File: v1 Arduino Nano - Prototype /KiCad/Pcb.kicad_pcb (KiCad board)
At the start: 2 copper layers, 4 parts

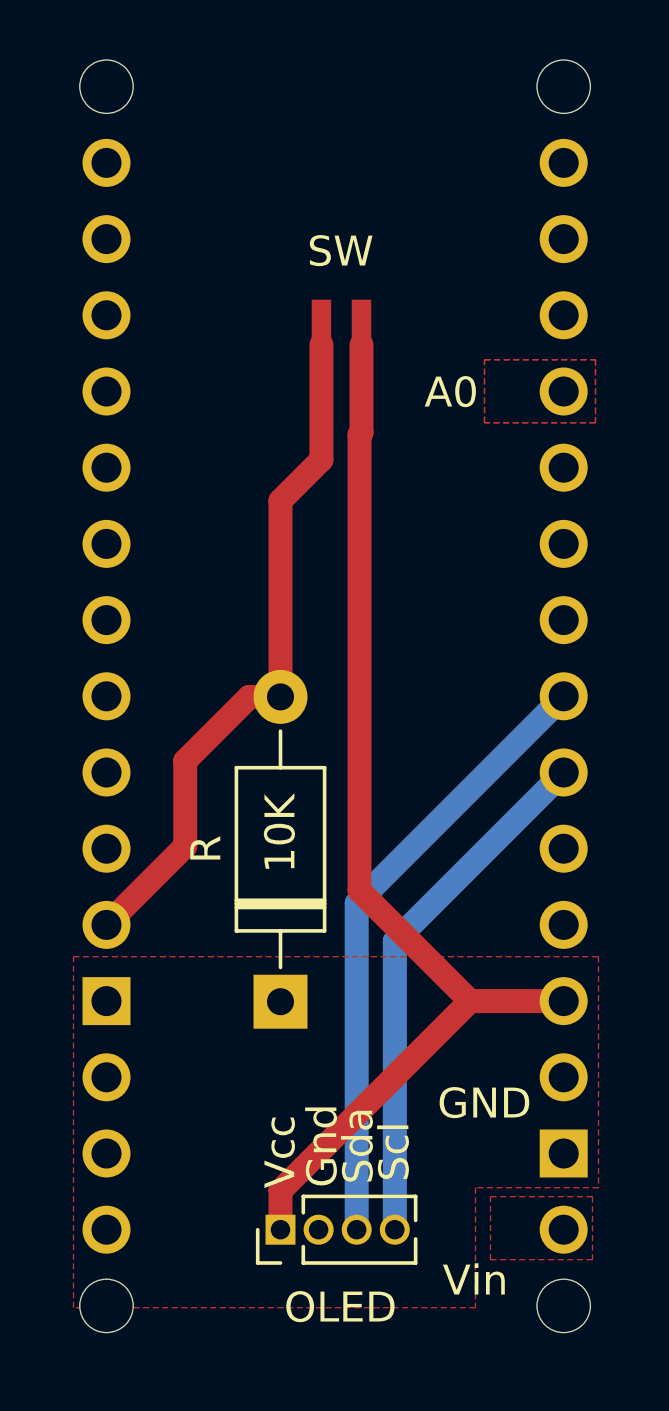
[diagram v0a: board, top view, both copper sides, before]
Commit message: update
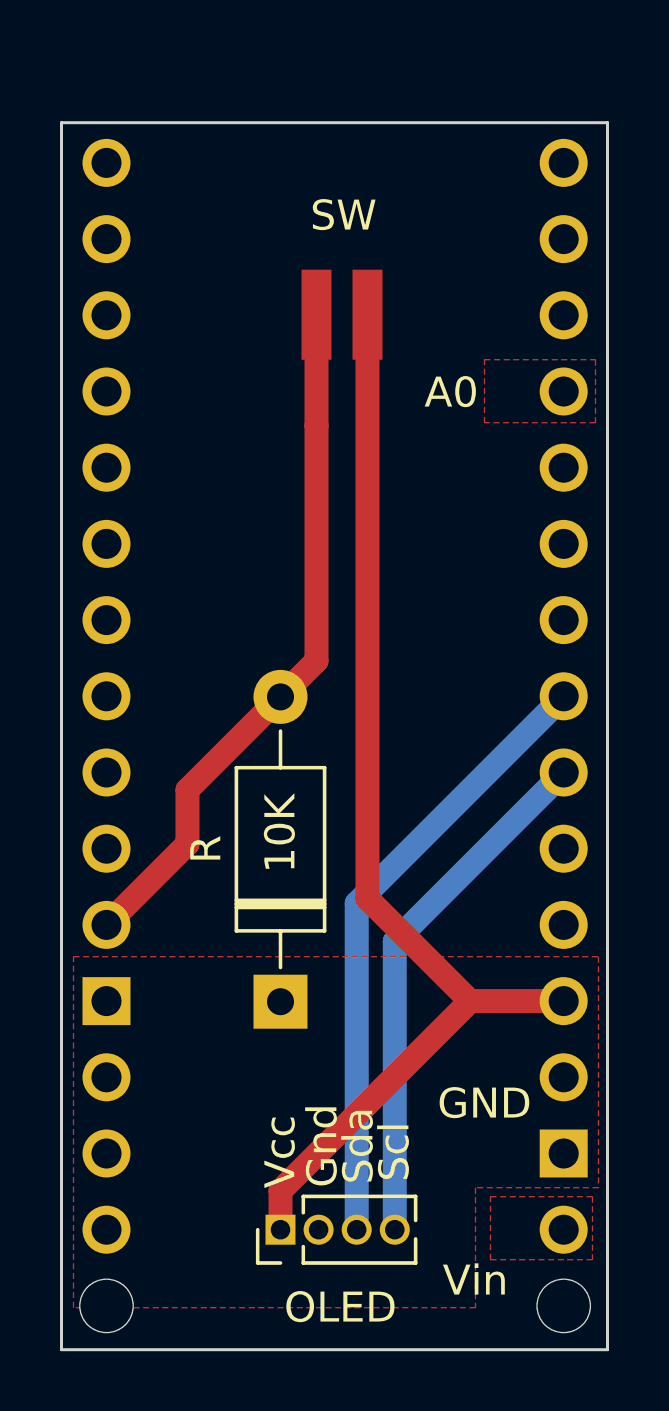
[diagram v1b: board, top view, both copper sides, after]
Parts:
- moved SW 4.00 mm to (180.7, 64.2), turned to -90 degrees
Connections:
- SW pad 1: Net-(A1-Pad5) -> /ARD5V
- SW pad 2: /ARD5V -> Net-(A1-Pad5)
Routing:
- net /ARD5V: track 36.8 -> 37.7 mm
- removed copper zone on F.Cu, net (none)
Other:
- board outline added: 18.2 x 40.9 mm
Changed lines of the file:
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@@
   )
   (module "Connector_PinHeader_1.27mm:PinHeader_1x02_P1.27mm_Vertical_SMD_Pin1Right" (layer "F.Cu")
-    (at 180.6 68.2 90)
+    (at 180.7 64.2 -90)
     (descr "surface-mounted straight pin header, 1x02, 1.27mm pitch, single row, style 2 (pin 1 right)")
     (tags "Surface mounted pin header SMD 1x02 1.27mm single row style2 pin1 right")
@@
     (property "Sheet name" "")
     (attr smd)
-    (fp_text reference "SW" (at 4.6 0) (layer "F.SilkS")
+    (fp_text reference "SW" (at -1.8 0) (layer "F.SilkS")
       (effects (font (size 1 1) (thickness 0.15)))
     )
@@
     (fp_line (start -3.5 1.8) (end 3.5 1.8) (layer "F.CrtYd") (width 0.05))
     (fp_line (start 3.5 1.8) (end 3.5 -1.8) (layer "F.CrtYd") (width 0.05))
+    (fp_line (start 3.5 -1.8) (end -3.5 -1.8) (layer "F.CrtYd") (width 0.05))
     (fp_line (start -3.5 -1.8) (end -3.5 1.8) (layer "F.CrtYd") (width 0.05))
-    (fp_line (start 3.5 -1.8) (end -3.5 -1.8) (layer "F.CrtYd") (width 0.05))
+    (fp_line (start 1.05 -0.835) (end 2.5 -0.835) (layer "F.Fab") (width 0.1))
+    (fp_line (start 2.5 -0.435) (end 1.05 -0.435) (layer "F.Fab") (width 0.1))
     (fp_line (start 2.5 -0.835) (end 2.5 -0.435) (layer "F.Fab") (width 0.1))
-    (fp_line (start 2.5 -0.435) (end 1.05 -0.435) (layer "F.Fab") (width 0.1))
-    (fp_line (start 1.05 -0.835) (end 2.5 -0.835) (layer "F.Fab") (width 0.1))
-    (pad "1" connect rect (at 1.5 -0.635 90) (size 3 0.65) (layers "F.Cu" "F.Mask")
-      (net 6 "Net-(A1-Pad5)") (pinfunction "1"))
-    (pad "2" connect rect (at 1.5 0.7 90) (size 3 0.65) (layers "F.Cu" "F.Mask")
-      (net 3 "/ARD5V") (pinfunction "2"))
+    (pad "1" connect rect (at 1.5 -0.8 270) (size 3 1) (layers "F.Cu" "F.Mask")
+      (net 3 "/ARD5V") (pinfunction "1"))
+    (pad "2" connect rect (at 1.5 0.9 270) (size 3 1) (layers "F.Cu" "F.Mask")
+      (net 6 "Net-(A1-Pad5)") (pinfunction "2"))
     (model "${KISYS3DMOD}/Connector_PinHeader_1.27mm.3dshapes/PinHeader_1x02_P1.27mm_Vertical_SMD_Pin1Right.wrl"
       (offset (xyz 0 0 0))
@@
     (property "Sheet name" "")
     (attr through_hole)
-    (fp_text reference "A1" (at 7.62 5.08) (layer "B.SilkS")
+    (fp_text reference "A1" (at 7.62 5.08) (layer "B.Fab")
       (effects (font (size 1 1) (thickness 0.15)) (justify mirror))
     )
@@
       (effects (font (size 1 1) (thickness 0.15)) (justify mirror))
     )
-    (fp_line (start -1.4 -1.27) (end -1.4 -39.5) (layer "B.SilkS") (width 0.12))
-    (fp_line (start 1.27 -36.83) (end -1.4 -36.83) (layer "B.SilkS") (width 0.12))
-    (fp_line (start -1.4 3.94) (end -1.4 1.27) (layer "B.SilkS") (width 0.12))
-    (fp_line (start 16.64 -39.5) (end 16.64 3.94) (layer "B.SilkS") (width 0.12))
-    (fp_line (start 13.97 -36.83) (end 16.64 -36.83) (layer "B.SilkS") (width 0.12))
-    (fp_line (start 1.27 -1.27) (end -1.4 -1.27) (layer "B.SilkS") (width 0.12))
-    (fp_line (start 16.64 3.94) (end -1.4 3.94) (layer "B.SilkS") (width 0.12))
-    (fp_line (start 13.97 1.27) (end 16.64 1.27) (layer "B.SilkS") (width 0.12))
-    (fp_line (start -1.4 -39.5) (end 16.64 -39.5) (layer "B.SilkS") (width 0.12))
-    (fp_line (start 1.27 -1.27) (end 1.27 -36.83) (layer "B.SilkS") (width 0.12))
-    (fp_line (start 1.27 1.27) (end -1.4 1.27) (layer "B.SilkS") (width 0.12))
-    (fp_line (start 13.97 1.27) (end 13.97 -36.83) (layer "B.SilkS") (width 0.12))
-    (fp_line (start 1.27 -1.27) (end 1.27 1.27) (layer "B.SilkS") (width 0.12))
-    (fp_line (start -1.53 4.06) (end -1.53 -42.16) (layer "B.CrtYd") (width 0.05))
+    (fp_line (start 16.75 -42.16) (end 16.75 4.06) (layer "B.CrtYd") (width 0.05))
     (fp_line (start 16.75 -42.16) (end -1.53 -42.16) (layer "B.CrtYd") (width 0.05))
     (fp_line (start -1.53 4.06) (end 16.75 4.06) (layer "B.CrtYd") (width 0.05))
-    (fp_line (start 16.75 -42.16) (end 16.75 4.06) (layer "B.CrtYd") (width 0.05))
-    (fp_line (start 16.51 3.81) (end 16.51 -39.37) (layer "B.Fab") (width 0.1))
+    (fp_line (start -1.53 4.06) (end -1.53 -42.16) (layer "B.CrtYd") (width 0.05))
+    (fp_line (start -1.27 -39.37) (end -1.27 2.54) (layer "B.Fab") (width 0.1))
+    (fp_line (start 3.81 -41.91) (end 3.81 -31.75) (layer "B.Fab") (width 0.1))
+    (fp_line (start -1.27 2.54) (end 0 3.81) (layer "B.Fab") (width 0.1))
     (fp_line (start 0 3.81) (end 16.51 3.81) (layer "B.Fab") (width 0.1))
     (fp_line (start 16.51 -39.37) (end -1.27 -39.37) (layer "B.Fab") (width 0.1))
     (fp_line (start 11.43 -31.75) (end 11.43 -41.91) (layer "B.Fab") (width 0.1))
-    (fp_line (start -1.27 -39.37) (end -1.27 2.54) (layer "B.Fab") (width 0.1))
+    (fp_line (start 16.51 3.81) (end 16.51 -39.37) (layer "B.Fab") (width 0.1))
+    (fp_line (start 11.43 -41.91) (end 3.81 -41.91) (layer "B.Fab") (width 0.1))
     (fp_line (start 3.81 -31.75) (end 11.43 -31.75) (layer "B.Fab") (width 0.1))
-    (fp_line (start -1.27 2.54) (end 0 3.81) (layer "B.Fab") (width 0.1))
-    (fp_line (start 3.81 -41.91) (end 3.81 -31.75) (layer "B.Fab") (width 0.1))
-    (fp_line (start 11.43 -41.91) (end 3.81 -41.91) (layer "B.Fab") (width 0.1))
-    (pad "" np_thru_hole circle (at 15.24 -38.1) (size 1.78 1.78) (drill 1.78) (layers *.Cu *.Mask))
+    (pad "" np_thru_hole circle (at 0 2.54) (size 1.78 1.78) (drill 1.78) (layers *.Cu *.Mask))
     (pad "" np_thru_hole circle (at 15.24 2.54) (size 1.78 1.78) (drill 1.78) (layers *.Cu *.Mask))
-    (pad "" np_thru_hole circle (at 0 2.54) (size 1.78 1.78) (drill 1.78) (layers *.Cu *.Mask))
-    (pad "" np_thru_hole circle (at 0 -38.1) (size 1.78 1.78) (drill 1.78) (layers *.Cu *.Mask))
     (pad "1" thru_hole oval (at 0 0) (size 1.6 1.6) (drill 1) (layers *.Cu *.Mask)
       (pinfunction "D1/RX"))
@@
     )
   )
+  (gr_rect (start 189.5 100.2) (end 171.3 59.3) (layer "Edge.Cuts") (width 0.1))
   (gr_text "10K" (at 178.6 83 90) (layer "F.SilkS")
     (effects (font (size 1 1) (thickness 0.15)))
@@
     (effects (font (size 1 1) (thickness 0.15)))
   )
-  (segment (start 181.235 84.895) (end 181.235 69.7) (width 0.8) (layer "F.Cu") (net 3))
   (segment (start 178.6 94.9) (end 184.92 88.58) (width 0.8) (layer "F.Cu") (net 3))
-  (segment (start 184.92 88.58) (end 181.235 84.895) (width 0.8) (layer "F.Cu") (net 3))
-  (segment (start 181.3 69.635) (end 181.3 66.7) (width 0.8) (layer "F.Cu") (net 3))
   (segment (start 184.92 88.58) (end 188.04 88.58) (width 0.8) (layer "F.Cu") (net 3))
+  (segment (start 181.5 65.7) (end 181.5 85.16) (width 0.8) (layer "F.Cu") (net 3))
   (segment (start 178.6 96.2) (end 178.6 94.9) (width 0.8) (layer "F.Cu") (net 3))
-  (segment (start 181.235 69.7) (end 181.3 69.635) (width 0.8) (layer "F.Cu") (net 3))
+  (segment (start 181.5 85.16) (end 184.92 88.58) (width 0.8) (layer "F.Cu") (net 3))
   (segment (start 182.41 96.2) (end 182.41 86.59) (width 0.8) (layer "B.Cu") (net 4))
   (segment (start 182.41 86.59) (end 188.04 80.96) (width 0.8) (layer "B.Cu") (net 4))
   (segment (start 181.14 96.2) (end 181.14 85.32) (width 0.8) (layer "B.Cu") (net 5))
   (segment (start 181.14 85.32) (end 188.04 78.42) (width 0.8) (layer "B.Cu") (net 5))
-  (segment (start 179.965 70.535) (end 179.965 66.7) (width 0.8) (layer "F.Cu") (net 6))
-  (segment (start 177.56 78.44) (end 178.6 78.44) (width 0.8) (layer "F.Cu") (net 6))
-  (segment (start 175.425 80.575) (end 177.56 78.44) (width 0.8) (layer "F.Cu") (net 6))
-  (segment (start 172.8 86.04) (end 175.425 83.415) (width 0.8) (layer "F.Cu") (net 6))
-  (segment (start 178.6 78.44) (end 178.6 71.9) (width 0.8) (layer "F.Cu") (net 6))
-  (segment (start 175.425 83.415) (end 175.425 80.575) (width 0.8) (layer "F.Cu") (net 6))
-  (segment (start 178.6 71.9) (end 179.965 70.535) (width 0.8) (layer "F.Cu") (net 6))
+  (segment (start 178.6 78.44) (end 175.5 81.54) (width 0.8) (layer "F.Cu") (net 6))
+  (segment (start 179.8 77.24) (end 178.6 78.44) (width 0.8) (layer "F.Cu") (net 6))
+  (segment (start 179.8 65.7) (end 179.8 69.4) (width 0.8) (layer "F.Cu") (net 6))
+  (segment (start 179.8 69.4) (end 179.8 77.24) (width 0.8) (layer "F.Cu") (net 6))
+  (segment (start 175.5 83.34) (end 172.8 86.04) (width 0.8) (layer "F.Cu") (net 6))
+  (segment (start 175.5 81.54) (end 175.5 83.34) (width 0.8) (layer "F.Cu") (net 6))
   (zone (net 1) (net_name "Net-(A1-Pad30)") (layer "F.Cu") (hatch edge 0.508)
     (connect_pads yes (clearance 0.508))
@@
     )
   )
-  (zone (net 0) (net_name "") (layer "F.Cu") (hatch edge 0.508)
-    (connect_pads yes (clearance 0.508))
-    (min_thickness 0.254) (filled_areas_thickness no)
-    (fill yes (thermal_gap 0.508) (thermal_bridge_width 0.508))
-    (polygon
-      (pts
-        (xy 189.1 69.3)
+  (zone (net 0) (net_name "") (layer "F.Mask") (hatch edge 0.508)
+    (connect_pads (clearance 0.508))
+    (min_thickness 0.254) (filled_areas_thickness no)
+    (fill yes (thermal_gap 0.508) (thermal_bridge_width 0.508) (smoothing fillet) (radius 0.5))
+    (polygon
+      (pts
+        (xy 189.2 69.3)
         (xy 185.4 69.3)
         (xy 185.4 67.2)
-        (xy 189.1 67.2)
-      )
-    )
+        (xy 189.2 67.2)
+      )
+    )
